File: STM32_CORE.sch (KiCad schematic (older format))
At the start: 31 parts, among them J6 Conn_01x14, J7 Conn_01x12, J8 Conn_01x12, SW1 SW_Push, U3 STM32F103C8T6, U4 AMS1117-3.3, Y1 O8M, Y2 O32.768K

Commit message: update,
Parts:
- Y1: footprint Crystal:Crystal_SMD_HC49-SD -> w_crystal:hc-49_smd
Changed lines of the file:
@@
 $Descr A3 16535 11693
 encoding utf-8
-Sheet 6 6
+Sheet 5 6
 Title ""
 Date ""
@@
 F 0 "Y1" V 14654 6788 50  0000 L CNN
 F 1 "O8M" V 14745 6788 50  0000 L CNN
-F 2 "Crystal:Crystal_SMD_HC49-SD" H 14700 6700 50  0001 C CNN
+F 2 "w_crystal:hc-49_smd" H 14700 6700 50  0001 C CNN
 F 3 "~" H 14700 6700 50  0001 C CNN
 	1    14700 6700

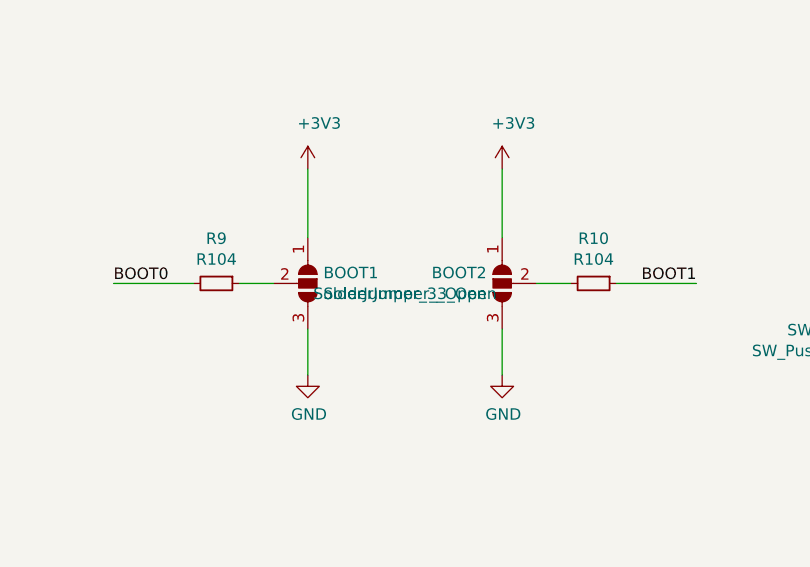
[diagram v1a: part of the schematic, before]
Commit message: update,
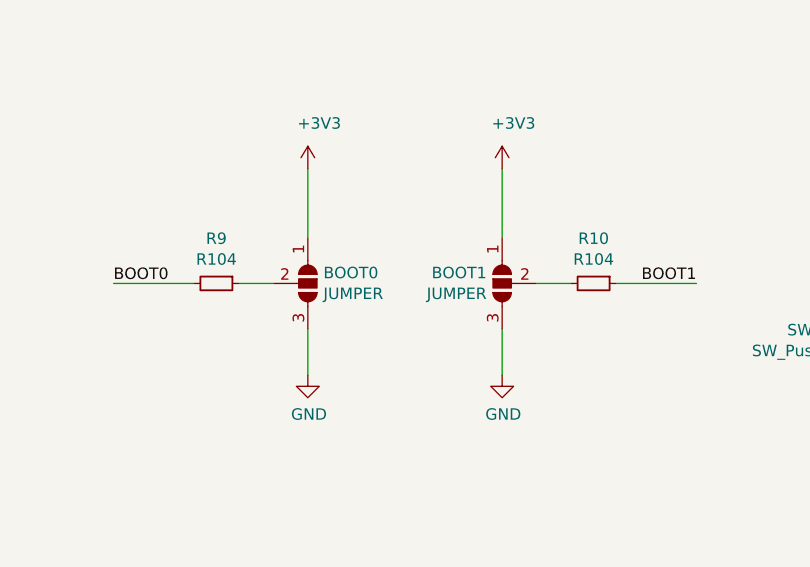
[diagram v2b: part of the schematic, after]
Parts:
- BOOT0: renamed from BOOT1; value SolderJumper_3_Open -> JUMPER
- BOOT1: renamed from BOOT2; value SolderJumper_3_Open -> JUMPER
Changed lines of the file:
@@
 	14500 3100 14500 3350
 $Comp
-L Jumper:SolderJumper_3_Open BOOT1
+L Jumper:SolderJumper_3_Open BOOT0
 U 1 1 5BCF8FA5
 P 11800 2850
-F 0 "BOOT1" V 11754 2918 50  0000 L CNN
-F 1 "SolderJumper_3_Open" V 11845 2918 50  0000 L CNN
+F 0 "BOOT0" V 11754 2918 50  0000 L CNN
+F 1 "JUMPER" V 11845 2918 50  0000 L CNN
 F 2 "Jumper:SolderJumper-3_P2.0mm_Open_TrianglePad1.0x1.5mm" H 11800 2850 50  0001 C CNN
 F 3 "~" H 11800 2850 50  0001 C CNN
@@
 $EndComp
 $Comp
-L Jumper:SolderJumper_3_Open BOOT2
+L Jumper:SolderJumper_3_Open BOOT1
 U 1 1 5BCF9021
 P 12650 2850
-F 0 "BOOT2" V 12604 2918 50  0000 L CNN
-F 1 "SolderJumper_3_Open" V 12695 2918 50  0000 L CNN
+F 0 "BOOT1" V 12604 2918 50  0000 L CNN
+F 1 "JUMPER" V 12695 2918 50  0000 L CNN
 F 2 "Jumper:SolderJumper-3_P2.0mm_Open_TrianglePad1.0x1.5mm" H 12650 2850 50  0001 C CNN
 F 3 "~" H 12650 2850 50  0001 C CNN
